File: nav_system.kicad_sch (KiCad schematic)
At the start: 16 parts, among them J1 GPS MODULE, J2 MPU6050, J3 SIM76003-L1C, J4 ESP32-CAM, J5 SW-420, J6 Conn_01x02_Socket, J7 SW-420 TOGGLE, J8 RGB, J9 RGB_GROUND, SW1 SW_SPDT

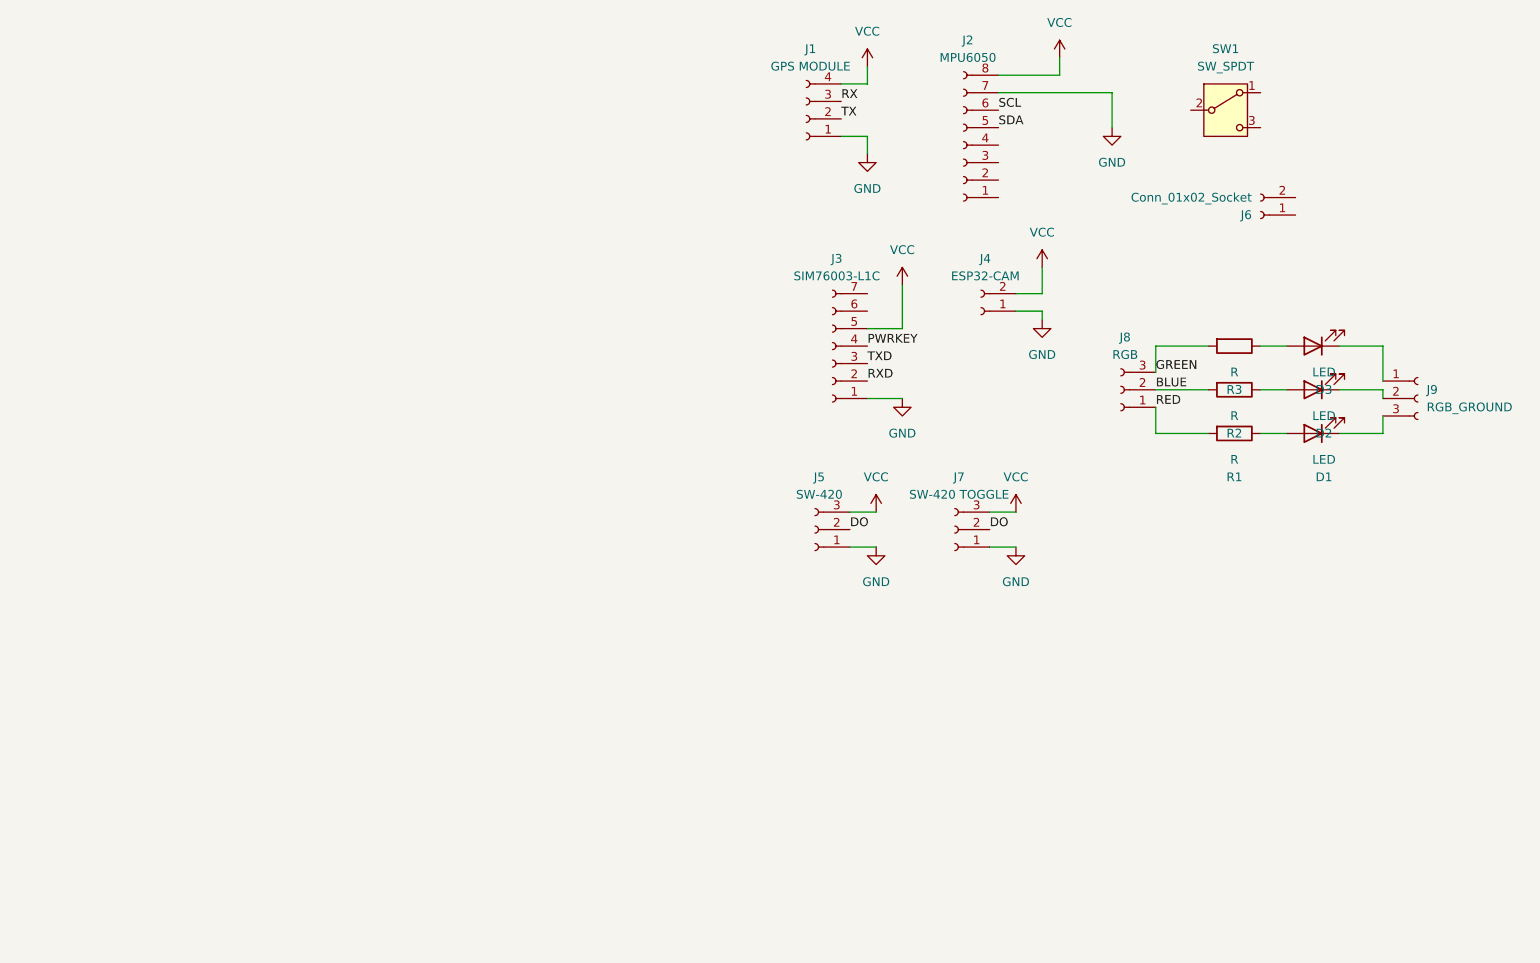
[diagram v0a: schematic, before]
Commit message: Trying to add 3d model
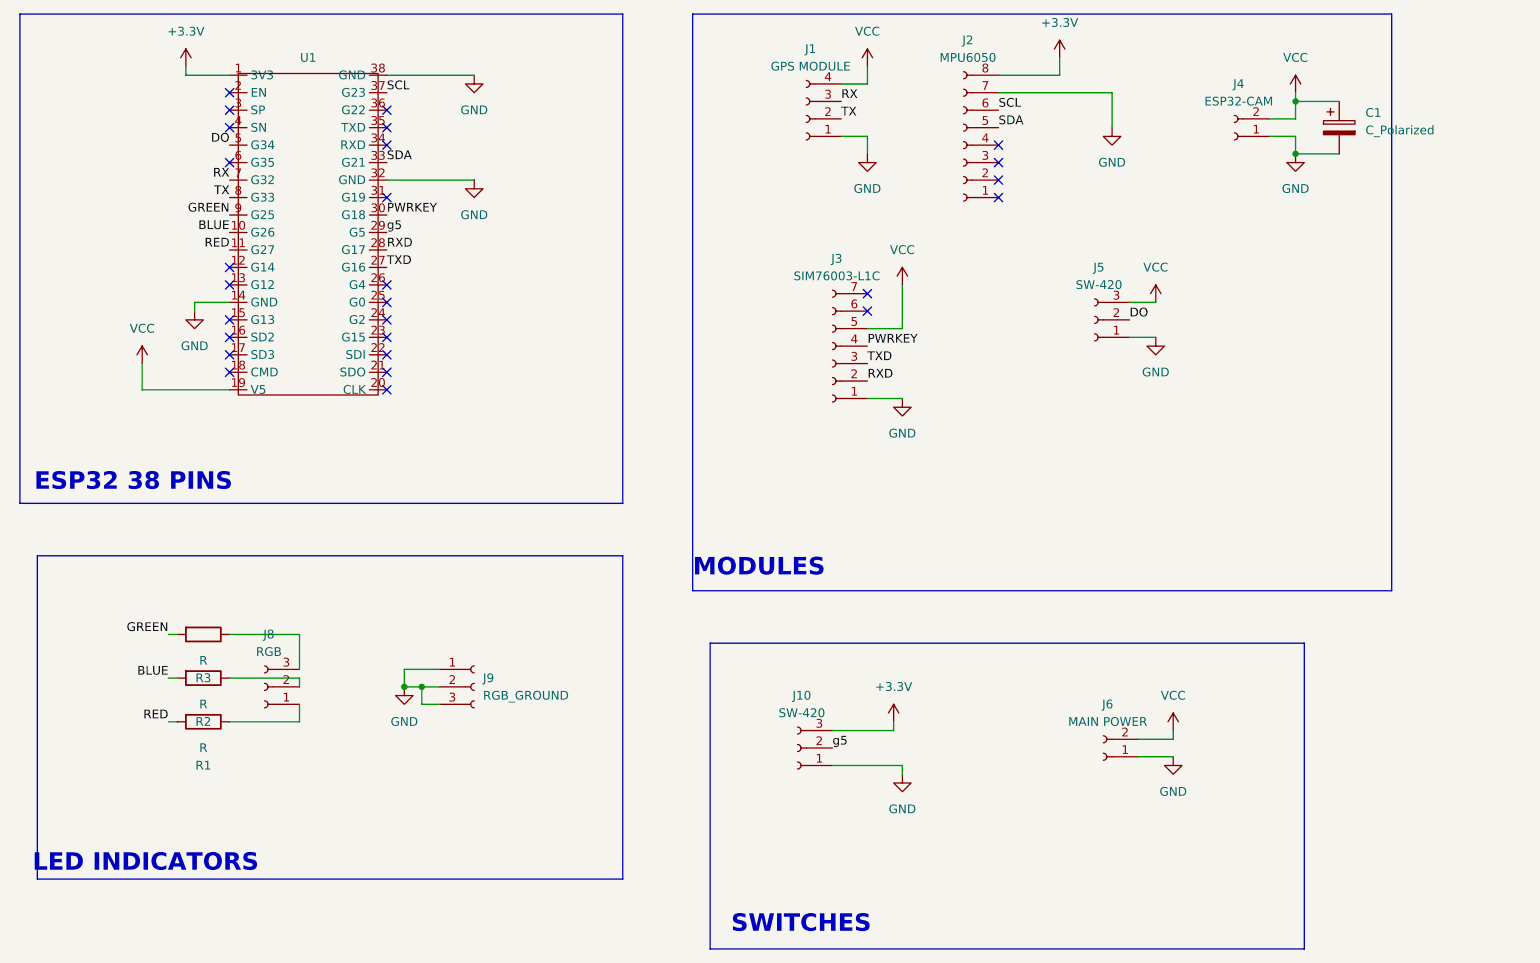
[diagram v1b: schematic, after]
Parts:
- removed D1, D2, D3: LED, symbol Device:LED
- removed J7: SW-420 TOGGLE, symbol Connector:Conn_01x03_Socket
- removed SW1: SW_SPDT, symbol Switch:SW_SPDT
- added C1: C_Polarized, Capacitor_THT:CP_Radial_D10.0mm_P3.50mm, symbol Device:C_Polarized
- added J10: SW-420, Connector_JST:JST_XH_B3B-XH-A_1x03_P2.50mm_Vertical, symbol Connector:Conn_01x03_Socket
- added U1: (no value), SHIELD:ESP32_38, symbol SHIELD:ESP32_38
- J1: footprint (none) -> Connector_PinSocket_2.54mm:PinSocket_1x04_P2.54mm_Vertical
- J2: footprint (none) -> Connector_PinSocket_2.54mm:PinSocket_1x08_P2.54mm_Vertical
- J3: footprint (none) -> Connector_PinSocket_2.54mm:PinSocket_1x07_P2.54mm_Vertical
- J4: footprint (none) -> Connector_JST:JST_XH_B2B-XH-A_1x02_P2.50mm_Vertical
- J5, J8, J9: footprint (none) -> Connector_JST:JST_XH_B3B-XH-A_1x03_P2.50mm_Vertical
- J6: value Conn_01x02_Socket -> MAIN POWER; footprint (none) -> Connector_JST:JST_XH_B2B-XH-A_1x02_P2.50mm_Vertical
- R1, R2, R3: footprint (none) -> Resistor_THT:R_Axial_DIN0204_L3.6mm_D1.6mm_P5.08mm_Horizontal
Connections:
- net BLUE: now also U1.10 (G26); no longer J8.2 (Pin_2)
- net DO: now also U1.5 (G34)
- net GND: now also J6.1 (Pin_1), J9.1 (Pin_1), J9.2 (Pin_2), J9.3 (Pin_3), C1.2, J10.1 (Pin_1), U1.14 (GND), U1.32 (GND), U1.38 (GND)
- net GREEN: now also U1.9 (G25); no longer J8.3 (Pin_3)
- net PWRKEY: now also U1.30 (G18)
- net RED: now also U1.11 (G27); no longer J8.1 (Pin_1)
- net RX: now also U1.7 (G32)
- net RXD: now also U1.28 (G17)
- net SCL: now also U1.37 (G23)
- net SDA: now also U1.33 (G21)
- net TX: now also U1.8 (G33)
- net TXD: now also U1.27 (G16)
- net VCC: now also J6.2 (Pin_2), C1.1, U1.19 (V5); no longer J2.8 (Pin_8)
- net at R2.1: now also J8.2 (Pin_2)
- net at R3.1: now also J8.3 (Pin_3)
- net at R1.1: now also J8.1 (Pin_1)
- new net +3.3V: J10.3 (Pin_3), J2.8 (Pin_8), U1.1 (3V3)
- new net g5: J10.2 (Pin_2), U1.29 (G5)
- no-connect marks 0 -> 27
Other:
- note added: "ESP32 38 PINS"
- note added: "LED INDICATORS"
- note added: "MODULES"
- note added: "SWITCHES"
- moved on the sheet: J4, J5, J6, J9, R1, R2, R3
